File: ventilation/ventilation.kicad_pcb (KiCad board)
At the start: 2 copper layers, 38 x 28.7 mm, 35 parts, among them J2 Conn_01x04_Pin, J3 Conn_01x04_Pin, J4 Conn_01x08_Pin, Q1 IRLML6402, Q2 BC847, U1 STM32L051C8Tx, U2 MCP1700x-330xxTT

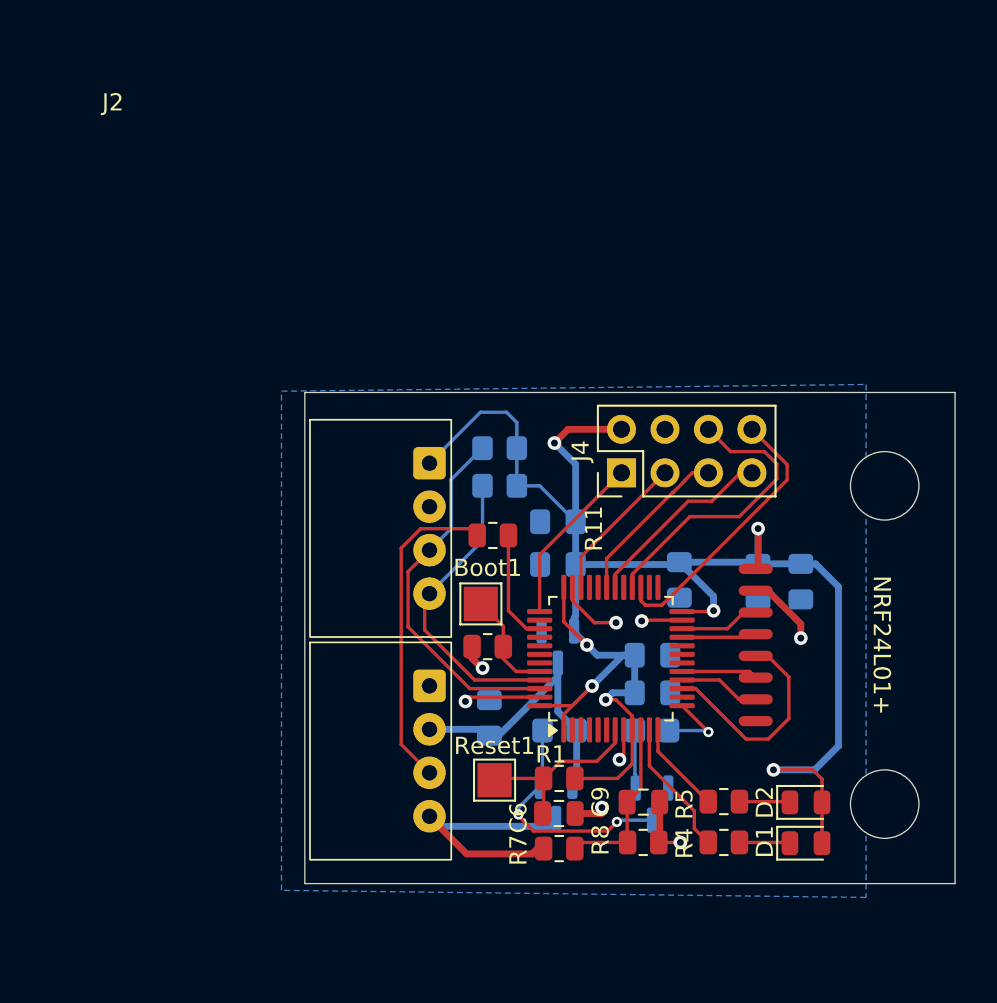
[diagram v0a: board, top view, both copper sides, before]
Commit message: New order
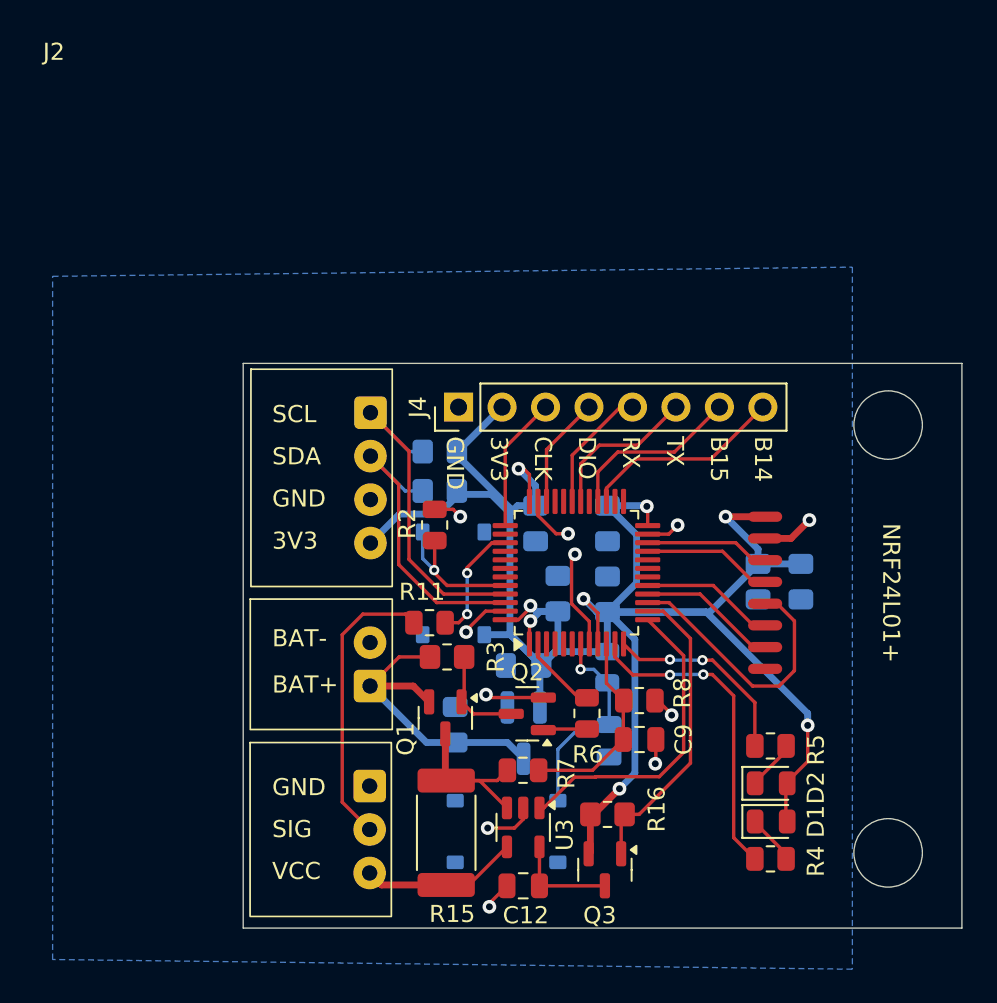
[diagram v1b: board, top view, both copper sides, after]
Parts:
- removed Boot1, Reset1: TestPoint, TestPoint:TestPoint_Pad_2.0x2.0mm
- removed J3: Conn_01x04_Pin, PVDW_custom:Connector_1x4_p2.54_hortizontal
- added BOOT1: SW_Push, PVDW_custom:SW_Push_4Pin, B.Cu at (166.2, 84.9)
- added C12: 10n, Capacitor_SMD:C_0805_2012Metric, F.Cu at (170.3, 102.6)
- added J1: Conn_01x02_Pin, PVDW_custom:Connector_1x2_p2.54_horizontal, F.Cu at (161.3, 90.9)
- added J5: Conn_01x03_Pin, PVDW_custom:Connector_1x3_p2.54_hortizontal, F.Cu at (161.3, 101.8)
- added Q3: IRLML6402, Package_TO_SOT_SMD:SOT-23, F.Cu at (175.1, 101.6)
- added R15: 0.1, Resistor_SMD:R_2512_6332Metric_Pad1.40x3.35mm_HandSolder, F.Cu at (165.8, 99.5)
- added R16: 10k, Resistor_SMD:R_0805_2012Metric_Pad1.20x1.40mm_HandSolder, F.Cu at (175.2, 98.4)
- added RESET1: SW_Push, PVDW_custom:SW_Push_4Pin, B.Cu at (169.3, 99.4)
- added U3: INA180A1, Package_TO_SOT_SMD:SOT-23-5, F.Cu at (170.3, 99.2)
- C6: value 100n -> 10n; moved to B.Cu
- J4: footprint Connector_PinHeader_2.54mm:PinHeader_2x04_P2.54mm_Vertical -> Connector_PinHeader_2.54mm:PinHeader_1x08_P2.54mm_Vertical
- Q1, Q2: moved to F.Cu
- R1: value 100k -> 10k; moved to B.Cu
- R3: value 40k -> 43k; moved to F.Cu
- R4: value 10k -> 1k2
- R5: value 10k -> 820
- R6: value 40k -> 43k; footprint Resistor_SMD:R_0805_2012Metric_Pad1.20x1.40mm_HandSolder -> Resistor_SMD:R_0805_2012Metric; moved to F.Cu
- R7: value 3k -> 3k3
- U2: footprint Package_TO_SOT_SMD:SOT-23 -> Package_TO_SOT_SMD:SOT-23_Handsoldering
- moved J4 10.3 mm to (166.5, 74.6)
- moved Q2 9.00 mm to (170.5, 92.5), turned to 180 degrees
- moved R8 8.29 mm to (177.1, 91.8)
- moved Q1 8.14 mm to (165.7, 92.8)
- moved R3 7.86 mm to (165.8, 89.2), turned to 180 degrees
- moved R2 7.76 mm to (165.1, 81.5), turned to 90 degrees
- moved R1 7.08 mm to (175.2, 89.8), turned to -90 degrees
- moved C3 6.60 mm to (172.3, 85.5), turned to 90 degrees
- moved C1 6.33 mm to (175.2, 85.5), turned to 90 degrees
- moved R11 6.30 mm to (164.8, 87.2)
- moved C11 6.23 mm to (170.3, 89.7)
- moved U1 5.41 mm to (173.4, 84.3)
- moved U2 5.41 mm to (170.3, 93.7)
- moved C4 5.34 mm to (175.2, 81.4)
- moved C6 5.17 mm to (175.3, 94.1), turned to -90 degrees
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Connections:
- net /VCC_SERVO renamed /SHUNT_P
- net Net-(D1-K) renamed /LED_RED_R
- net Net-(D2-K) renamed /LED_GREEN_R
- J2 pad 1: +3V3 -> /I2C_SCL
- J2 pad 2: GND -> /I2C_SDA
- J2 pad 3: /I2C_SDA -> GND
- J2 pad 4: /I2C_SCL -> +3V3
- J4 pad 1: /SWCLK -> GND
- J4 pad 3: /SWDIO -> /SWCLK
- J4 pad 4: GND -> /SWDIO
- J4 pad 6: /PB15 -> /USART1_TX
- J4 pad 7: /USART1_TX -> /PB15
- U1 pad 13: /SW_SERVO -> /INA_OUT
- U1 pad 14: unconnected-(U1-PA4-Pad14) -> /SW_I_SERVO
- U1 pad 2: unconnected-(U1-PC13-Pad2) -> /SW_SERVO
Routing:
- net +3V3: track 107.8 -> 129.4 mm, vias 7 -> 8
- net /INA_OUT: track 0.00 -> 18.4 mm
- net /SW_I_SERVO: track 0.00 -> 17.9 mm
- net /LED_RED: track 8.00 -> 18.7 mm, vias 0 -> 2
- net /SHUNT_N: track 0.00 -> 9.24 mm
- net /G_FET: track 13.9 -> 5.88 mm, vias 2 -> 0
- net /PB15: track 17.2 -> 10.4 mm
- net /LED_GREEN: track 5.41 -> 11.6 mm, vias 0 -> 2
- net /INA_VCC: track 0.00 -> 6.10 mm
- net GND: track 23.9 -> 29.4 mm, vias 8 -> 11
- net /SHUNT_P: track 15.7 -> 10.8 mm
- net /PB14: track 16.3 -> 11.9 mm
- net /SPI_MOSI: track 4.45 -> 7.83 mm
- net /SPI_MISO: track 4.77 -> 8.15 mm
- net /I2C_SDA: track 21.4 -> 18.1 mm
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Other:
- board size 38 x 28.7 mm -> 42 x 33 mm
- board text added: "3V3"
- board text added: "B14"
- board text added: "B15"
- board text added: "BAT+"
- board text added: "BAT-"
- board text added: "CLK"
- board text added: "DIO"
- board text added: "GND"
- board text added: "PVDW 2025"
- board text added: "RX"
- board text added: "SCL"
- board text added: "SDA"
- board text added: "SIG"
- board text added: "TX"
- board text added: "VCC"
